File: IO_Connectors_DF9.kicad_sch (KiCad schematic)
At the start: 6 parts, among them U1 NX1H35 PBGA625, U11 AS4C8M16SA-6BIN

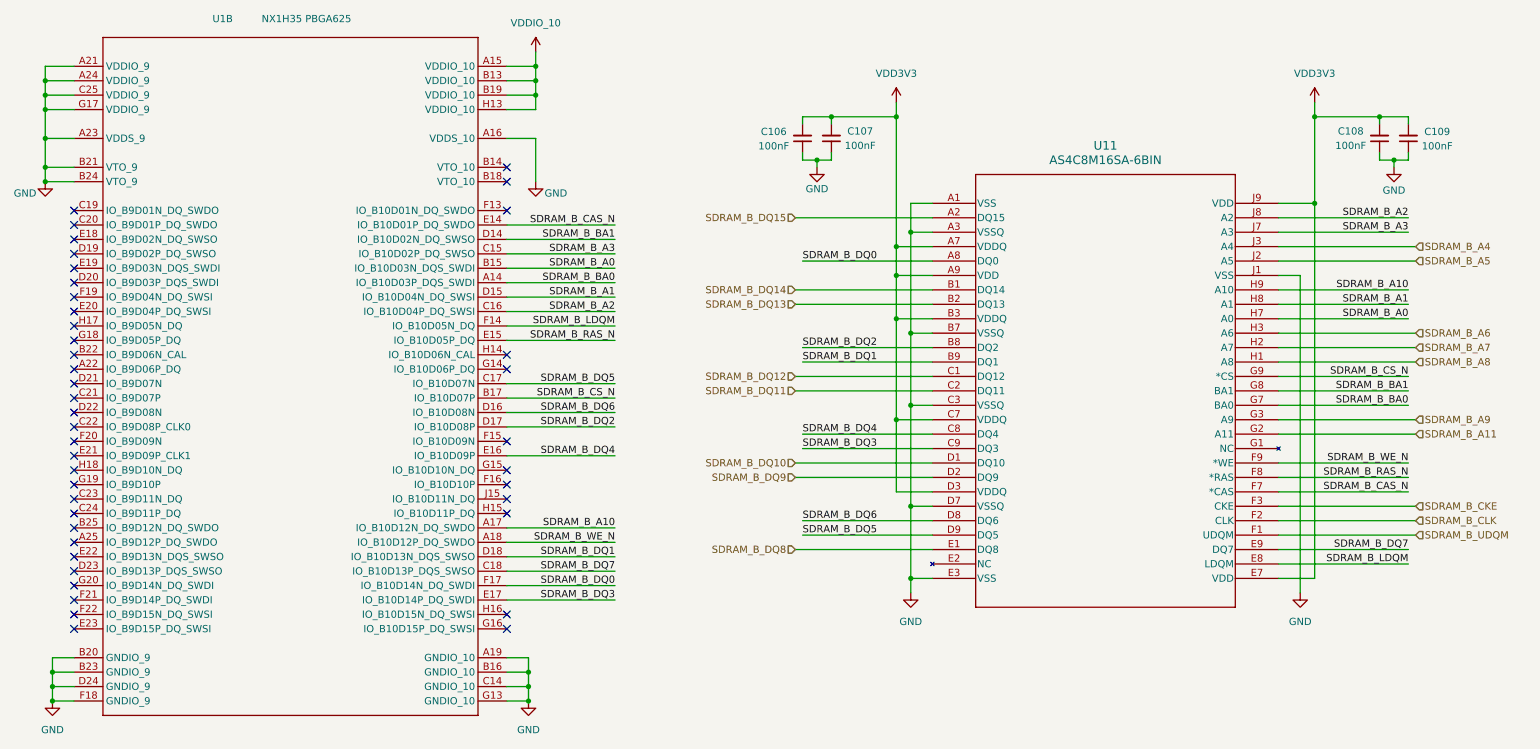
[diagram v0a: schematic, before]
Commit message: power tree
power tree defined. Few changes remaining but almost finalized
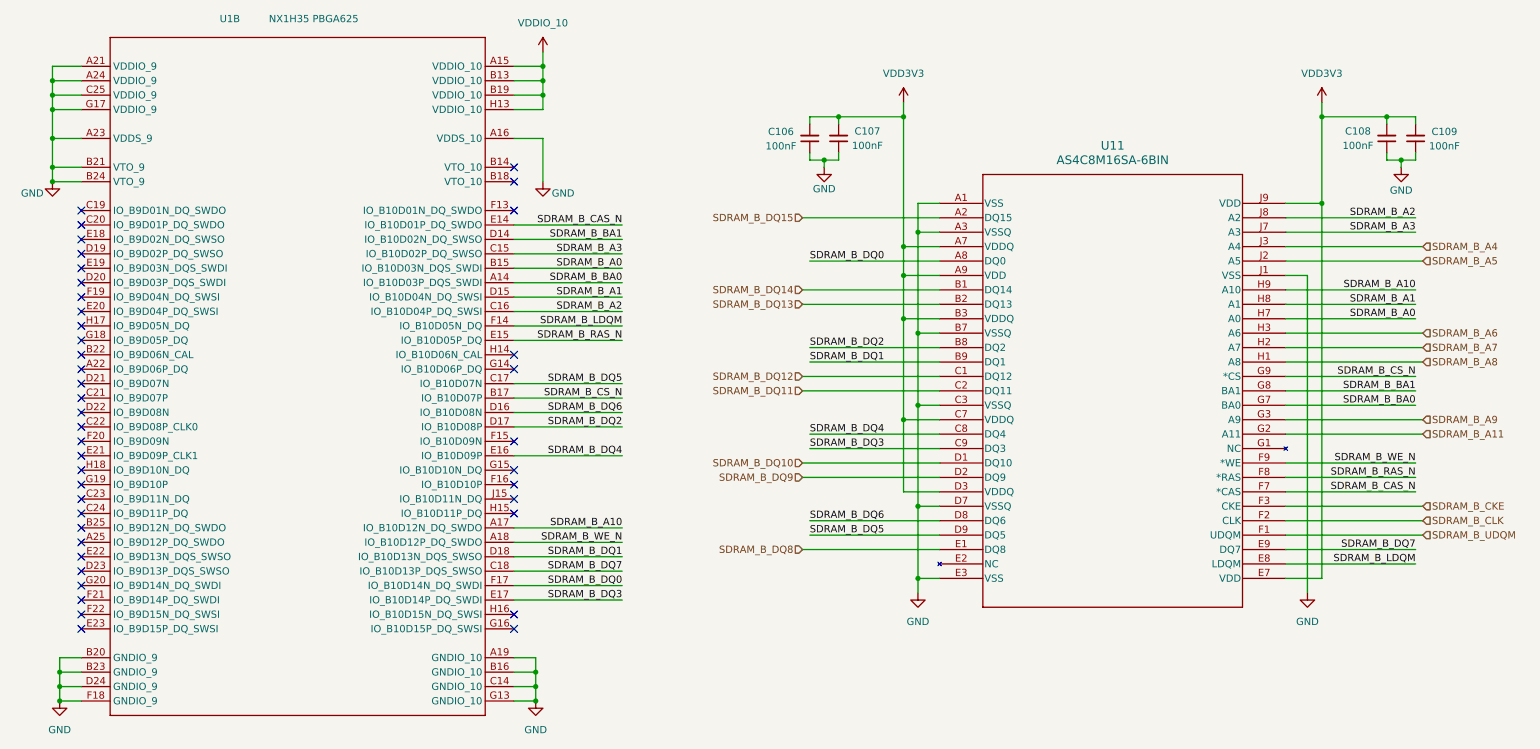
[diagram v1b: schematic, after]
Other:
- moved on the sheet: C106, C107, C108, C109, U11, U1B
